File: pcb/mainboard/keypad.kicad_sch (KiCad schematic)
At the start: 8 parts

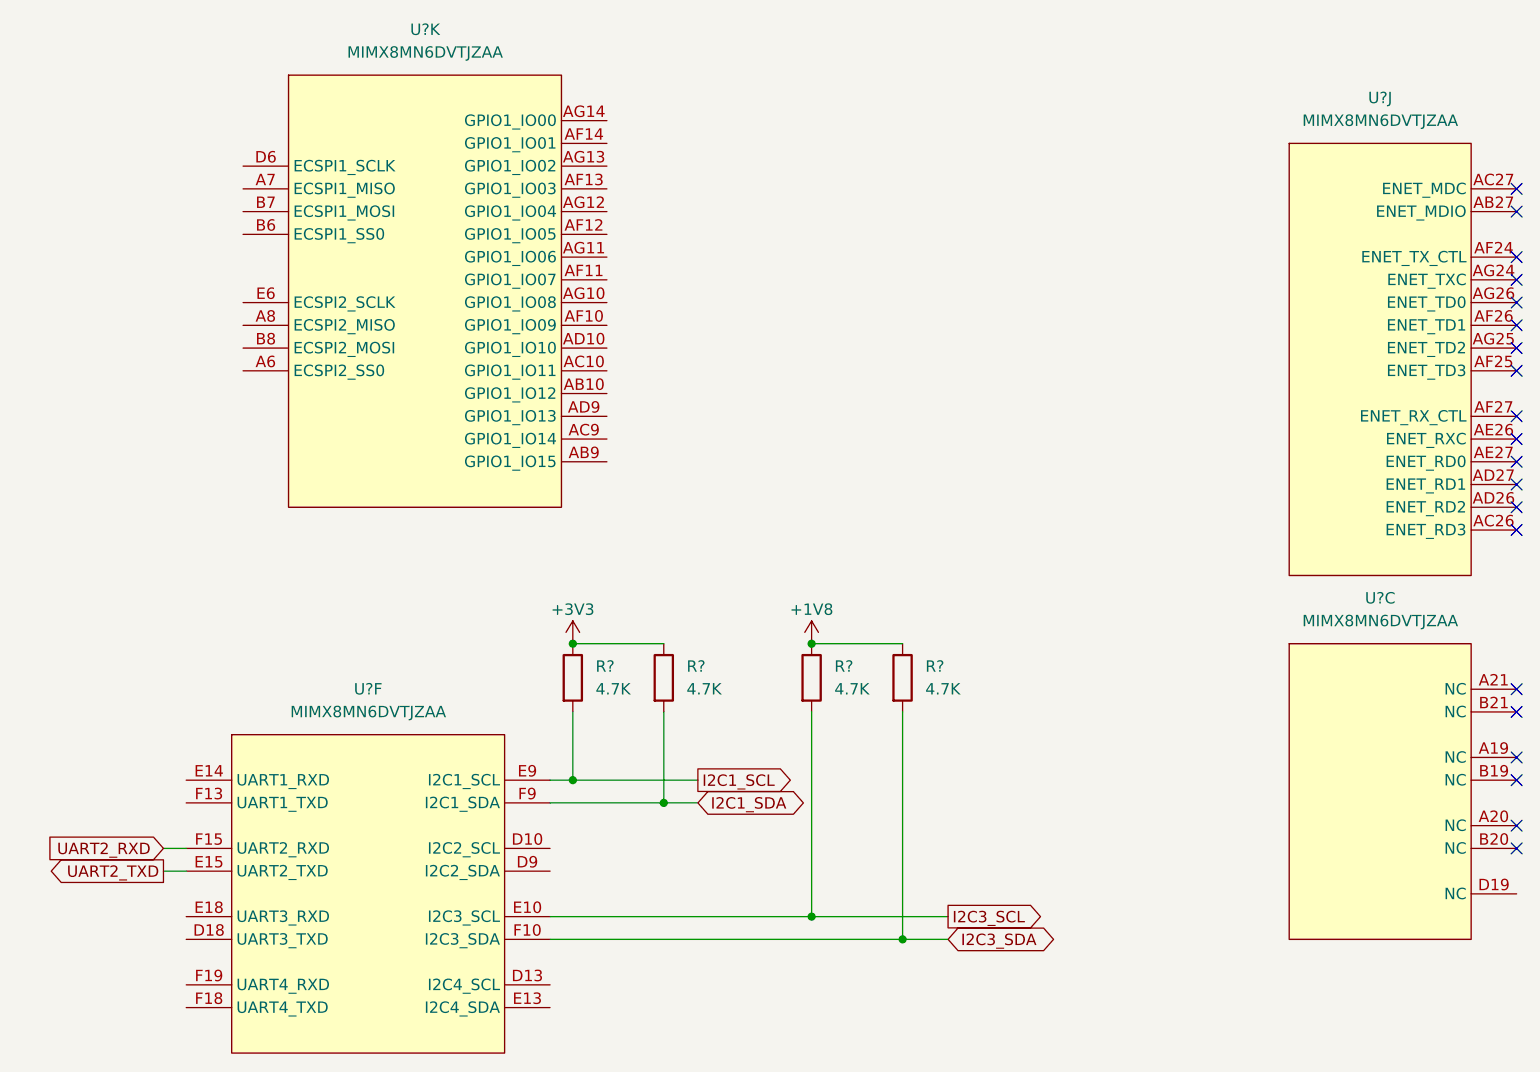
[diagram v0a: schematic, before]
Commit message: Working on mainboard schematics
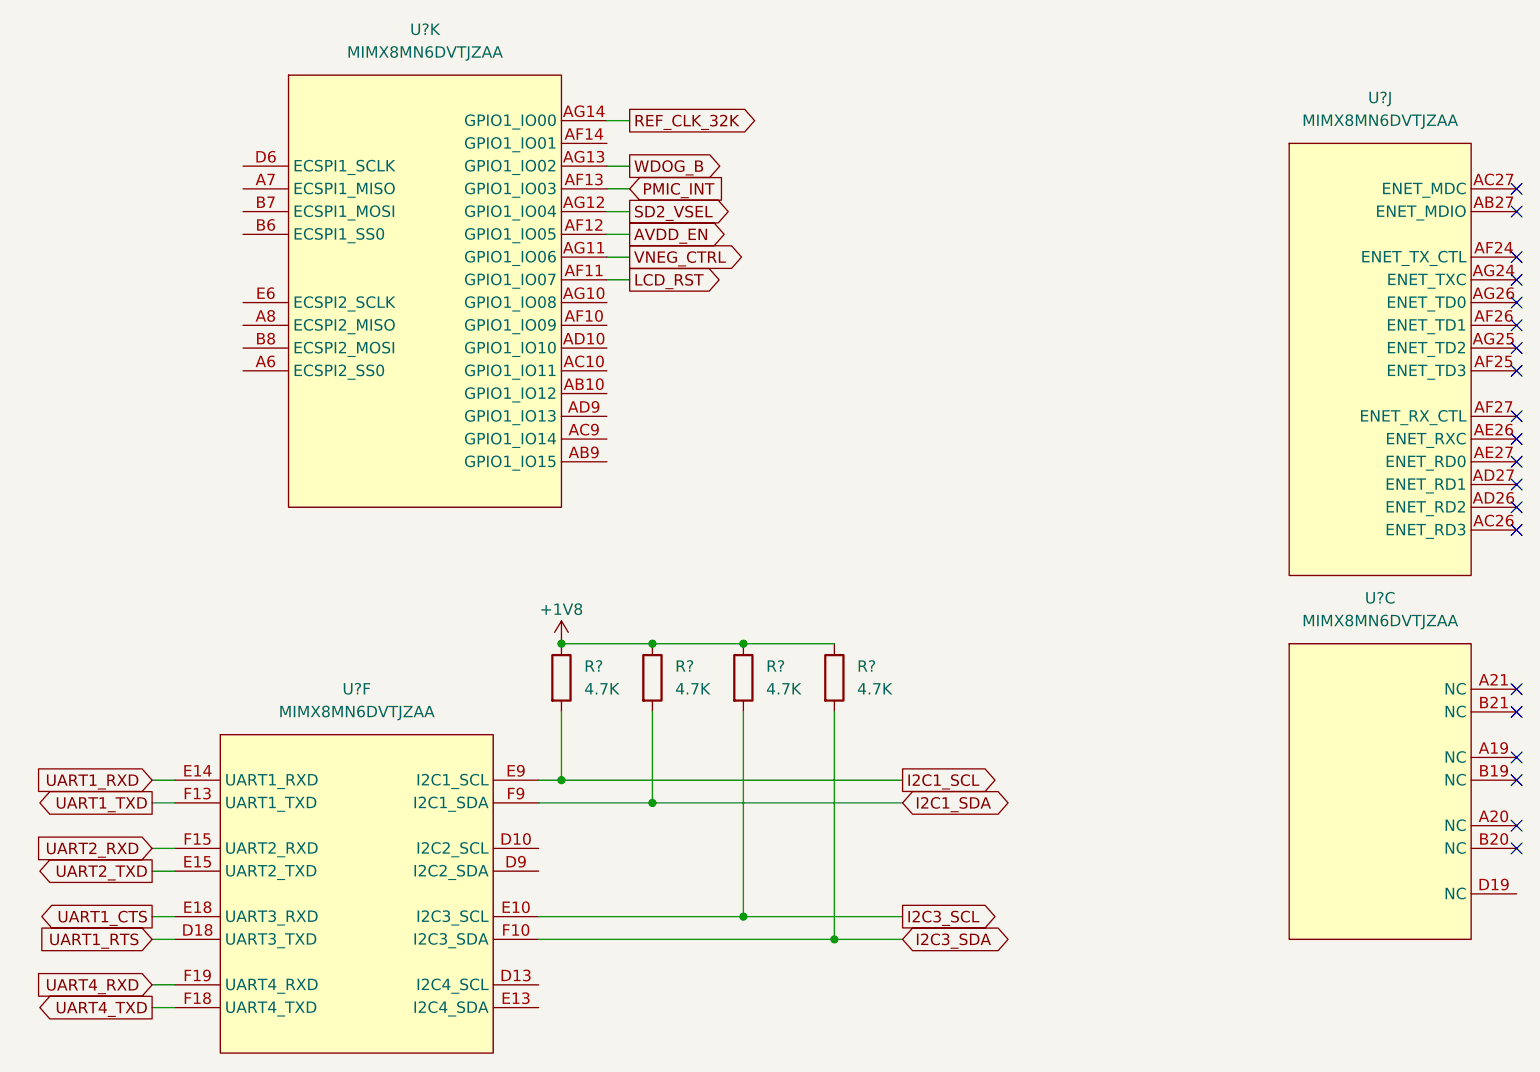
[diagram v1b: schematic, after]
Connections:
- net +3V3 is gone; now on net +1V8: R?.1, R?.1
- net LCD_RST: now reaches U?.AF11 (GPIO1_IO07)
- net AVDD_EN: now reaches U?.AF12 (GPIO1_IO05)
- net PMIC_INT: now reaches U?.AF13 (GPIO1_IO03)
- net VNEG_CTRL: now reaches U?.AG11 (GPIO1_IO06)
- net SD2_VSEL: now reaches U?.AG12 (GPIO1_IO04)
- net WDOG_B: now reaches U?.AG13 (GPIO1_IO02)
- net REF_CLK_32K: now reaches U?.AG14 (GPIO1_IO00)
- net UART1_RTS: now reaches U?.D18 (UART3_TXD)
- net UART1_RXD: now reaches U?.E14 (UART1_RXD)
- net UART1_CTS: now reaches U?.E18 (UART3_RXD)
- net UART1_TXD: now reaches U?.F13 (UART1_TXD)
- net UART4_TXD: now reaches U?.F18 (UART4_TXD)
- net UART4_RXD: now reaches U?.F19 (UART4_RXD)
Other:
- moved on the sheet: R?, U?F
